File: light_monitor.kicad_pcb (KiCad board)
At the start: 2 copper layers, 33.8 x 33.8 mm, 19 parts, among them IC1 TSL25911FN, J1 Conn_01x03, U1 STM32L432KCUx, U2 STDC14, U5 RV-8803-C7

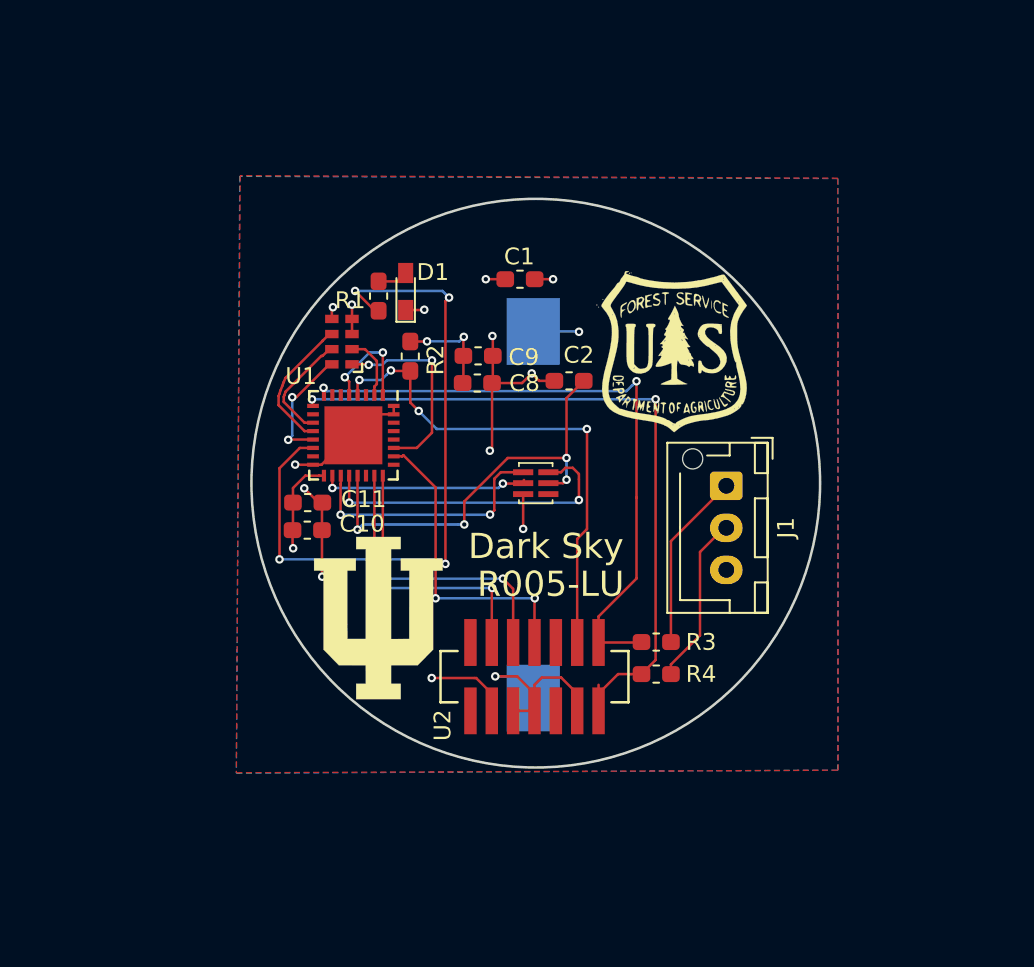
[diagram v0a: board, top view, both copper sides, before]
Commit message: r006 sensor committed
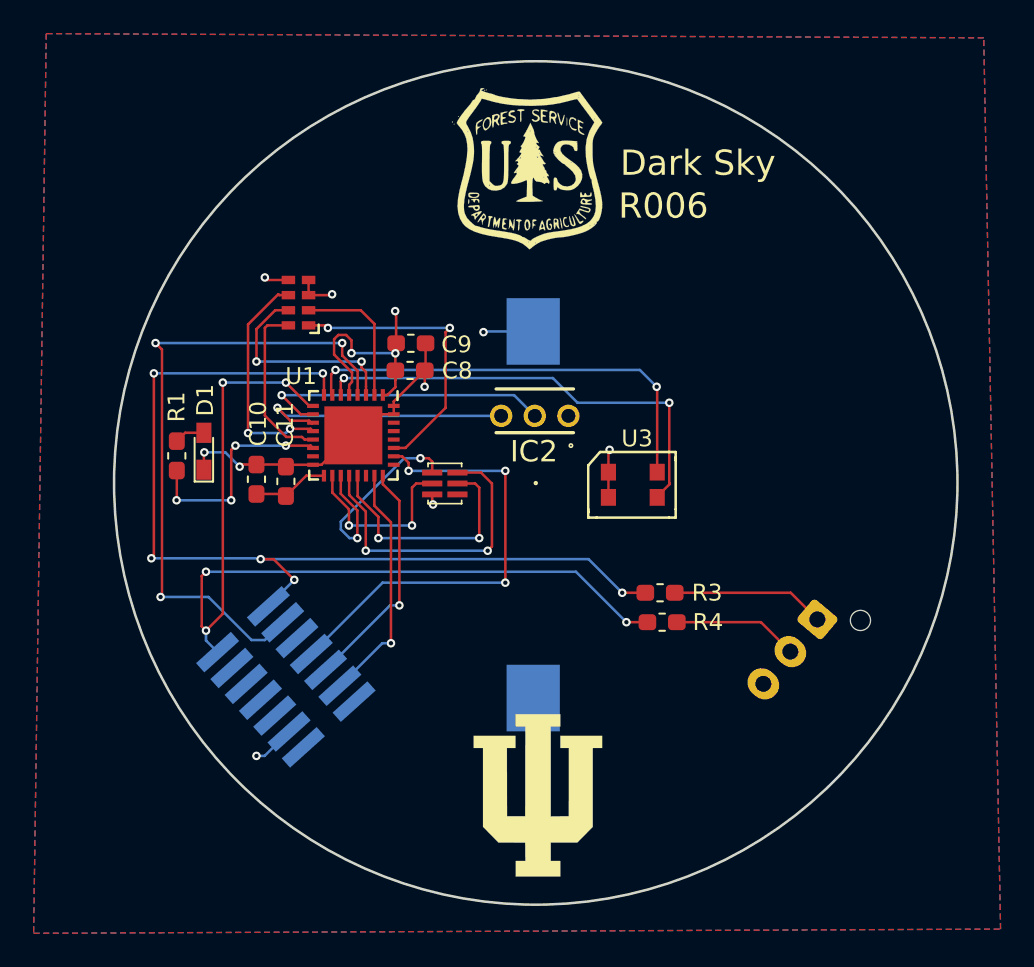
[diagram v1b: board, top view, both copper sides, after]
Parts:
- removed C1: 10uF, Capacitor_SMD:C_0603_1608Metric_Pad1.05x0.95mm_HandSolder
- removed C2: 0.1uF, Capacitor_SMD:C_0603_1608Metric_Pad1.05x0.95mm_HandSolder
- removed G30: LOGO, logo:hnf_logo
- removed G31: LOGO, logo:iu_trident
- removed R2: 100k, Resistor_SMD:R_0603_1608Metric_Pad1.05x0.95mm_HandSolder
- added G***: LOGO, logo:iu_trident, F.Cu at (113.5, 123.8)
- added G***: LOGO, logo:hnf_logo, F.Cu at (113.0, 86.5)
- added IC2: TSL237S-LF, SamacSys_Parts_3:TSL237S-LF, F.Cu at (113.3, 101.2)
- added U3: sm_tsl237, bhimebau_lightsensor:tsl237t, F.Cu at (119.8, 102.5)
- J1, U2: moved to B.Cu
- moved D1 15.3 mm to (93.6, 103.3)
- moved R1 15.3 mm to (92.0, 103.6)
- moved U2 14.8 mm to (98.5, 116.8), turned to 132 degrees
- moved J1 9.62 mm to (130.1, 113.3), turned to 230 degrees
- moved IC1 5.41 mm to (108.0, 105.3)
- moved C10 4.28 mm to (96.8, 105.0), turned to 90 degrees
- moved C8 4.07 mm to (105.9, 98.5)
- moved C9 4.07 mm to (105.9, 96.9)
- moved U5 3.47 mm to (99.2, 94.5)
- moved R4 3.11 mm to (120.9, 113.5)
- moved R3 2.94 mm to (120.8, 111.8)
- moved C11 1.81 mm to (98.5, 105.1), turned to 90 degrees
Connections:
- U1 pad 10: (no net) -> /tsl237_pwr
- U1 pad 11: /rtc_EVI -> /tsl237_freq
- U1 pad 3: (no net) -> /rtc_EVI
- U1 pad 6: (no net) -> /sm_237t_pwr
- U1 pad 7: (no net) -> /sm_237t_freq
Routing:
- net Net-(R1-Pad1): track 41.5 -> 13.0 mm
- net /sm_237t_pwr: track 0.00 -> 27.0 mm, vias 0 -> 2
- net /sm_237t_freq: track 0.00 -> 26.2 mm, vias 0 -> 2
- net /TX: track 38.4 -> 57.4 mm, vias 2 -> 6
- net /tsl237_pwr: track 0.00 -> 17.9 mm, vias 0 -> 1
- net GND: track 45.8 -> 29.4 mm, vias 11 -> 6
- net /tsl237_freq: track 0.00 -> 16.0 mm, vias 0 -> 1
- net /sensor_power: track 25.8 -> 14.6 mm, vias 4 -> 2
- net /RX: track 43.1 -> 53.9 mm, vias 2 -> 5
- net /SWO: track 18.6 -> 27.2 mm, vias 2 -> 3
- net /NRST: track 30.2 -> 38.6 mm, vias 4 -> 3
- net /rtc_EVI: track 6.68 -> 12.6 mm, vias 0 -> 2
- net /rtc_data: track 11.8 -> 17.4 mm
- net /rtc_nINT: track 8.22 -> 13.6 mm, vias 0 -> 2
- net /oscillator: track 3.85 -> 8.47 mm
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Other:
- board size 33.8 x 33.8 mm -> 50.2 x 50.2 mm
- board text added: "R006"
- board text removed: "R005-LU"
